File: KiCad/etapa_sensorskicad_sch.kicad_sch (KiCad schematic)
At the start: 4 parts, among them U6 FDC2214

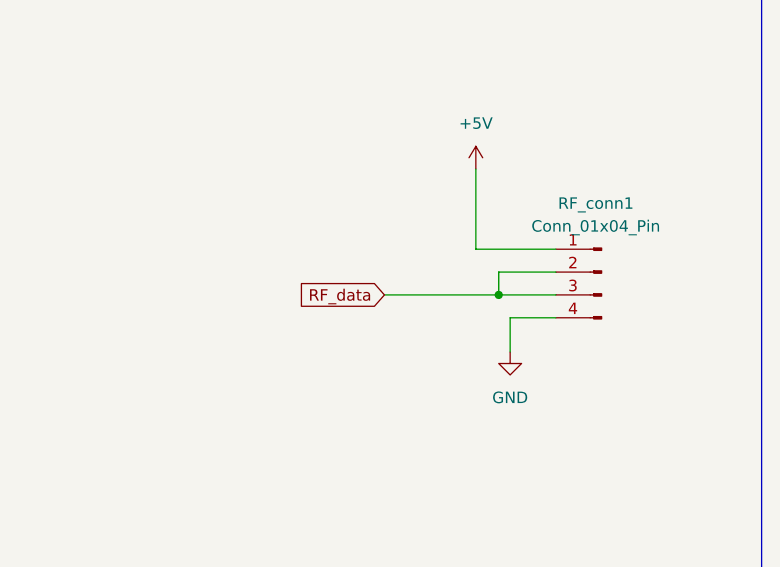
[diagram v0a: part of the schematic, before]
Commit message: Nose broderk
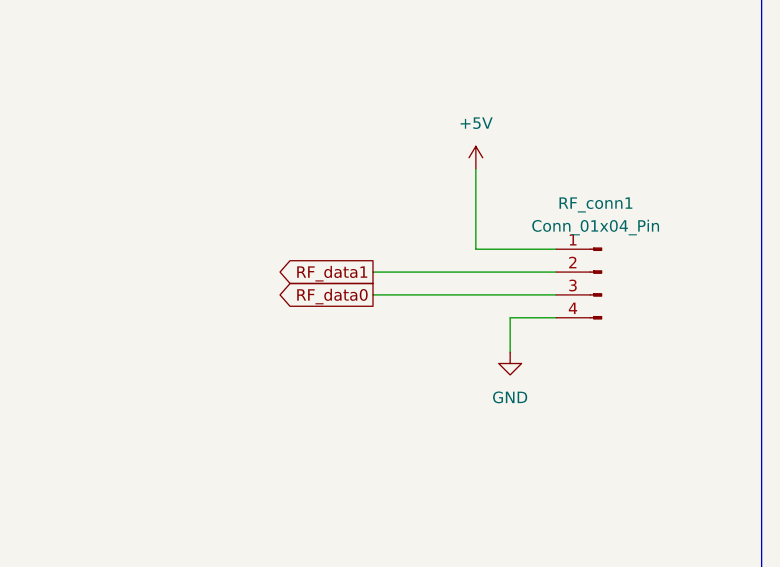
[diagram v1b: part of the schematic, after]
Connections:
- net RF_data renamed RF_data0
- net RF_data0: no longer RF_conn1.2 (Pin_2)
- new net RF_data1: RF_conn1.2 (Pin_2)
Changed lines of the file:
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@@
 		(color 0 0 0 0)
 	)
-	(junction
-		(at 144.78 63.5)
-		(diameter 0)
-		(color 0 0 0 0)
-	)
 	(no_connect
 		(at 31.75 64.77)
@@
 	(wire
 		(pts
-			(xy 144.78 60.96) (xy 144.78 63.5)
-		)
-		(stroke
-			(width 0)
-			(type default)
-		)
-	)
-	(wire
-		(pts
 			(xy 146.05 66.04) (xy 146.05 69.85)
 		)
@@
 	(wire
 		(pts
+			(xy 130.81 60.96) (xy 151.13 60.96)
+		)
+		(stroke
+			(width 0)
+			(type default)
+		)
+	)
+	(wire
+		(pts
 			(xy 31.75 68.58) (xy 24.13 68.58)
 		)
@@
 	(wire
 		(pts
-			(xy 132.08 63.5) (xy 144.78 63.5)
+			(xy 130.81 63.5) (xy 151.13 63.5)
 		)
 		(stroke
@@
 	(wire
 		(pts
-			(xy 151.13 60.96) (xy 144.78 60.96)
-		)
-		(stroke
-			(width 0)
-			(type default)
-		)
-	)
-	(wire
-		(pts
 			(xy 31.75 57.15) (xy 24.13 57.15)
 		)
@@
 		(pts
 			(xy 19.05 74.93) (xy 31.75 74.93)
-		)
-		(stroke
-			(width 0)
-			(type default)
-		)
-	)
-	(wire
-		(pts
-			(xy 144.78 63.5) (xy 151.13 63.5)
 		)
 		(stroke
@@
 		)
 	)
+	(global_label "RF_data1"
+		(shape output)
+		(at 130.81 60.96 180)
+		(fields_autoplaced yes)
+		(effects
+			(font
+				(size 1.27 1.27)
+			)
+			(justify right)
+		)
+		(property "Intersheetrefs" "${INTERSHEET_REFS}"
+			(at 119.1164 60.96 0)
+			(effects
+				(font
+					(size 1.27 1.27)
+				)
+				(justify right)
+				(hide yes)
+			)
+		)
+	)
 	(global_label "SDA"
 		(shape bidirectional)
@@
 		)
 	)
-	(global_label "RF_data"
-		(shape input)
-		(at 132.08 63.5 180)
+	(global_label "RF_data0"
+		(shape output)
+		(at 130.81 63.5 180)
 		(fields_autoplaced yes)
 		(effects
@@
 		)
 		(property "Intersheetrefs" "${INTERSHEET_REFS}"
-			(at 121.5959 63.5 0)
+			(at 119.1164 63.5 0)
 			(effects
 				(font
